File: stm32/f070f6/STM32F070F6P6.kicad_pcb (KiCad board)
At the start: 2 copper layers, 20.3 x 33.5 mm, 27 parts, among them J1 STLINK, J2 USB_C_REC_16PIN, J3 L, J4 L, SW1 BOOT0, U1 XC6220B331MR, U2 STM32F070F6Px, Y1 8 MHz

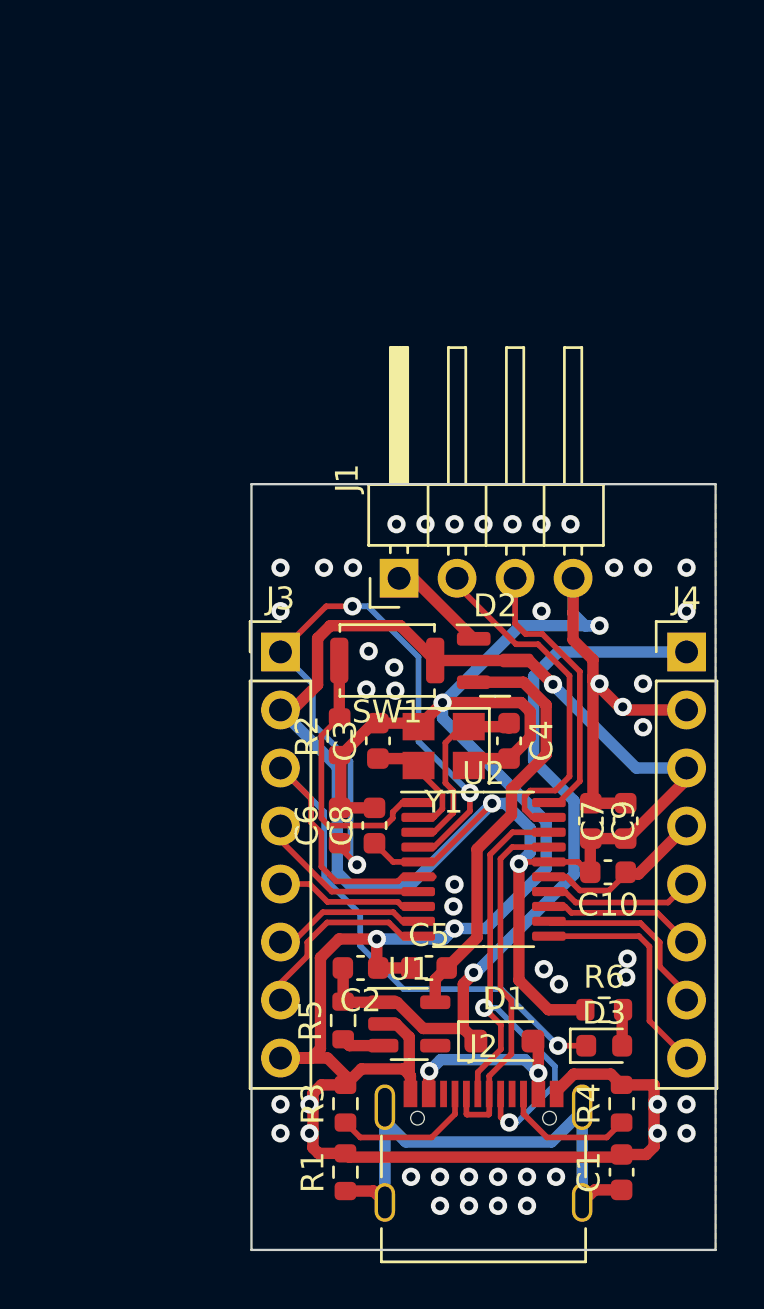
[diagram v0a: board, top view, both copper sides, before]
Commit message: Update 2023-11-27
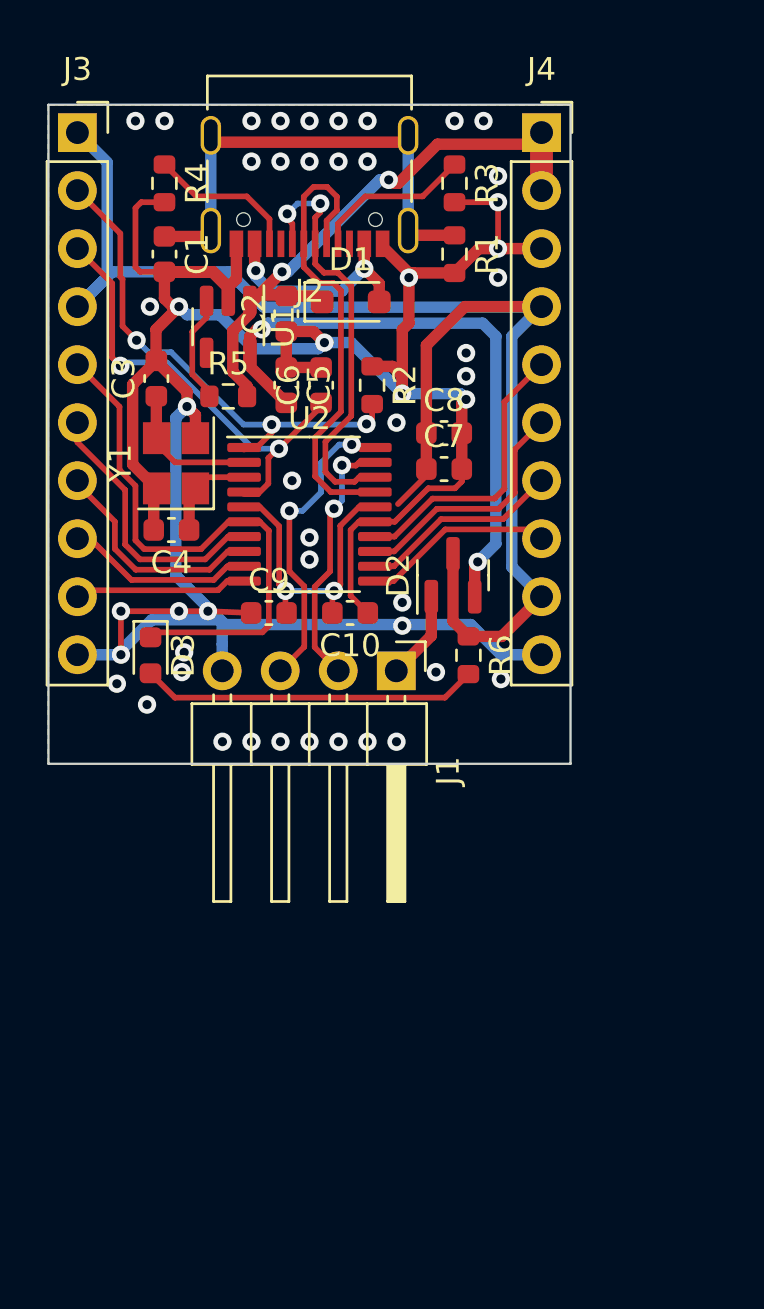
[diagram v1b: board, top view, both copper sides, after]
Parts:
- removed SW1: BOOT0, Button_Switch_SMD:SW_Push_SPST_NO_Alps_SKRK
- J3, J4: footprint Connector_PinHeader_2.54mm:PinHeader_1x08_P2.54mm_Vertical -> Connector_PinSocket_2.54mm:PinSocket_1x10_P2.54mm_Vertical
- moved R4 45.0 mm to (30.5, 26.4), turned to -90 degrees
- moved C1 44.9 mm to (30.5, 29.5), turned to -90 degrees
- moved J2 42.9 mm to (36.8, 26.5), turned to 180 degrees
- moved R3 40.6 mm to (43.2, 26.4), turned to -90 degrees
- moved R1 40.5 mm to (43.2, 29.5), turned to -90 degrees
- moved D1 33.1 mm to (38.6, 31.5)
- moved U1 31.5 mm to (33.3, 32.6), turned to -90 degrees
- moved C2 28.8 mm to (35.8, 32.1), turned to 90 degrees
- moved R5 27.8 mm to (33.3, 35.7), turned to 0 degrees
- moved C5 26.3 mm to (35.8, 35.2), turned to -90 degrees
- moved D3 26.2 mm to (29.9, 47.0), turned to -90 degrees
- moved J3 24.4 mm to (26.7, 24.1)
- moved J4 23.6 mm to (47.0, 24.1)
- moved C6 19.3 mm to (37.3, 35.2)
- moved C3 18.6 mm to (30.1, 34.9)
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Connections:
- J3 pad 1: NRST -> +3.3V
- J3 pad 2: +3.3V -> BOOT0
- J3 pad 3: PA0 -> NRST
- J3 pad 4: PA1 -> +3.3V
- J3 pad 5: PA2 -> PA0
- J3 pad 6: PA3 -> PA1
- J3 pad 7: PA4 -> PA2
- J3 pad 8: GND -> PA3
- J4 pad 2: GND -> +5V
- J4 pad 3: +3.3V -> GND
- J4 pad 4: GND -> +3.3V
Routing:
- net Net-(D3-A): track 1.59 -> 14.8 mm
- net +3.3V: track 69.5 -> 79.6 mm, vias 3 -> 2
- net NRST: track 30.4 -> 20.3 mm, vias 3 -> 2
- net BOOT0: track 12.2 -> 22.3 mm, vias 0 -> 3
- net +3.3VA: track 18.6 -> 26.6 mm, vias 0 -> 2
- net GND: track 121.4 -> 128.8 mm, vias 52 -> 50
- net +5V: track 33.4 -> 26.6 mm, vias 1 -> 2
- net PA0: track 31.3 -> 25.0 mm, vias 1 -> 0
- net PB1: track 6.56 -> 12.6 mm
- net USB_DM: track 16.0 -> 20.7 mm
- net PA1: track 7.59 -> 12.1 mm
- net USB_DP: track 23.2 -> 18.8 mm
- net PA7: track 6.67 -> 10.7 mm
- net SWDIO: track 15.4 -> 11.4 mm, vias 0 -> 2
- net HSE_OUT: track 8.22 -> 4.27 mm
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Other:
- board size 20.3 x 33.5 mm -> 22.9 x 28.9 mm
